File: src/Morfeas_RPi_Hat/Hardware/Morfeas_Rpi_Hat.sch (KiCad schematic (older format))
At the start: 53 parts, among them J1 Con, J2 RPi_header, J5 RS_232, Q1 SUM110P06, Q2 SUM110P06, U1 DS3231, U2 TSR2-2450, U3 TLV70433, U4 SP3232, U5 24AA08, U6 MAX9611, U7 MAX9611

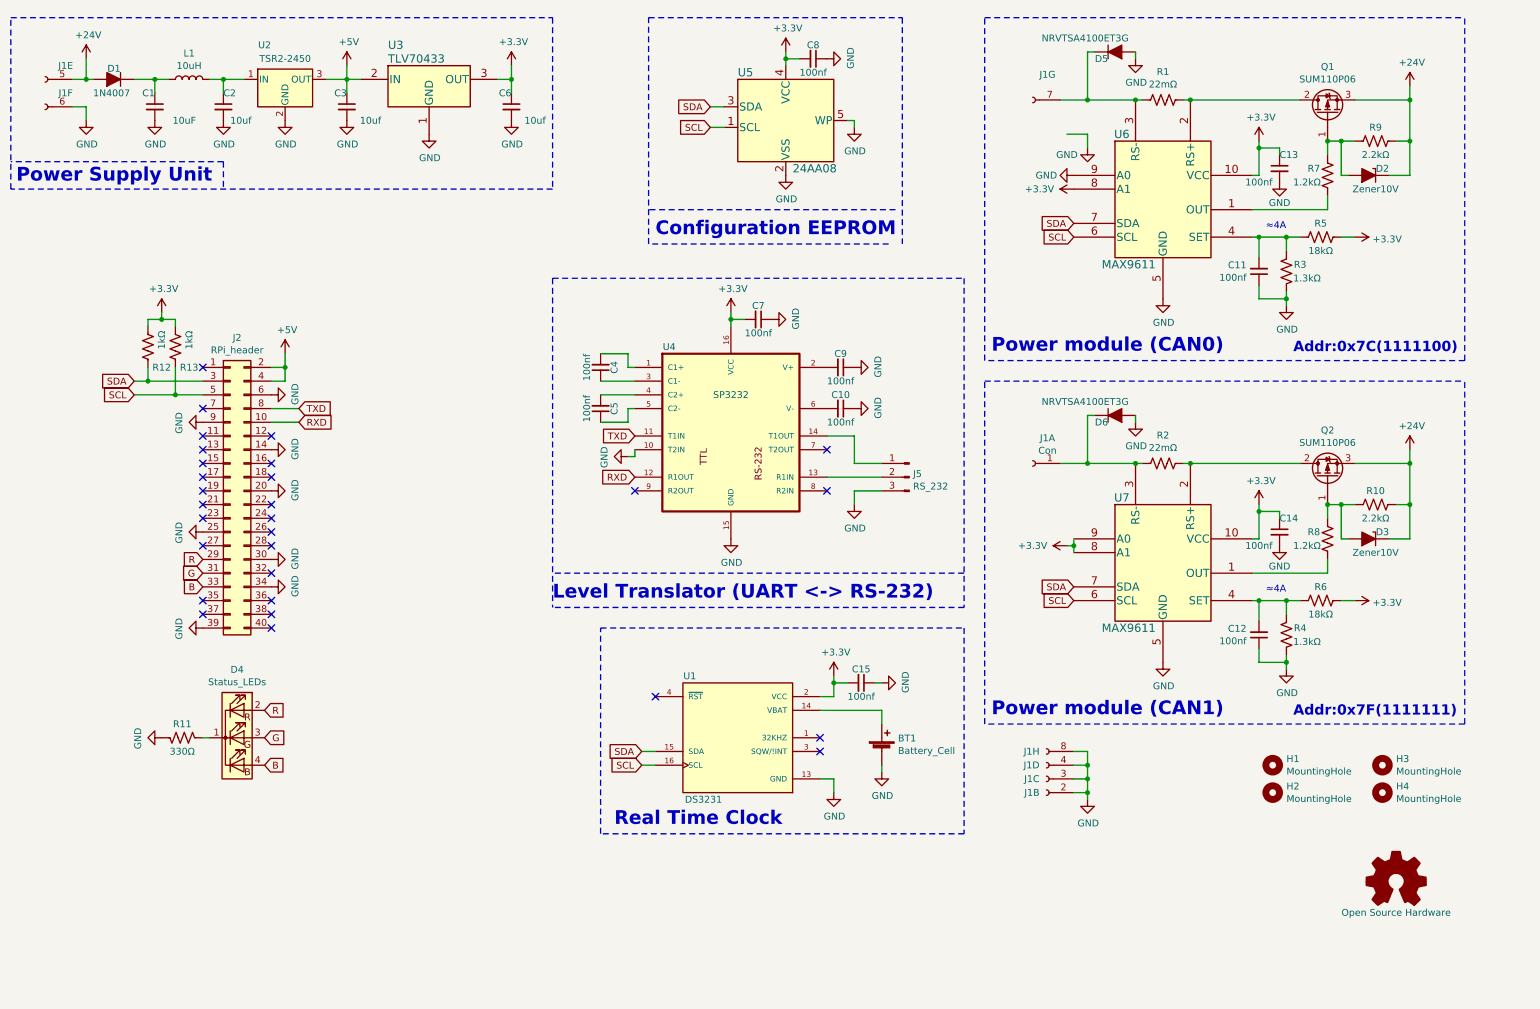
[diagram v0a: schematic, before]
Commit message: Update Morfeas_RPi_Hat
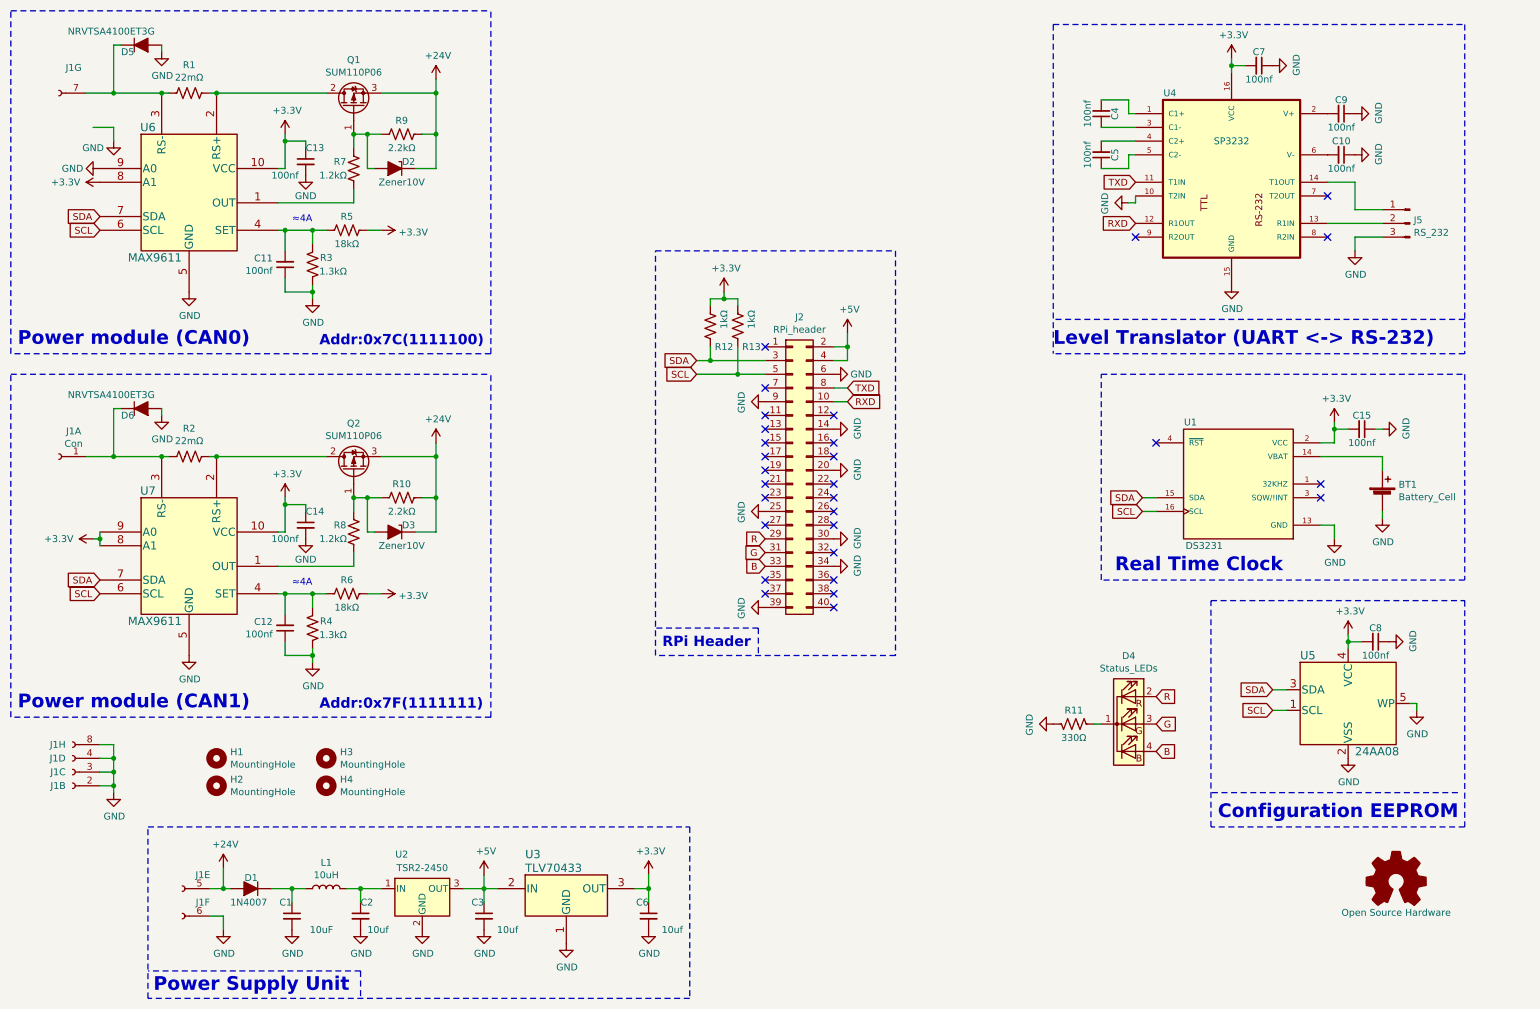
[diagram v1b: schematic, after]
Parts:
- D1: footprint Diode_THT:D_DO-41_SOD81_P10.16mm_Horizontal -> Morfeas_RPi_hat:DO-214AC(SMA)
- L1: footprint Inductor_THT:L_Axial_L6.6mm_D2.7mm_P10.16mm_Horizontal_Vishay_IM-2 -> Resistors_SMD:R_2816_HandSoldering
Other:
- note added: "RPi Header"
- moved on the sheet: BT1, C1, C10, C11, C12, C13, C14, C15, C2, C3, C4, C5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
